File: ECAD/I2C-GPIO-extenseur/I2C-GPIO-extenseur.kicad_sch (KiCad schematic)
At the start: 61 parts, among them J1 Conn_01x03, J10 Conn_01x03, J11 Conn_01x03, J12 Conn_01x03, J13 Conn_01x03, J14 Conn_01x03, J15 Conn_01x03, J16 Conn_01x03, J17 Conn_01x03, J18 Conn_01x04, J19 Conn_01x04, J2 Conn_01x02, J3 Conn_01x03, J4 Conn_01x03, J5 Conn_01x03, J6 Conn_01x03, J7 Conn_01x03, J8 Conn_01x03, J9 Conn_01x03, U1 PCA9685PW

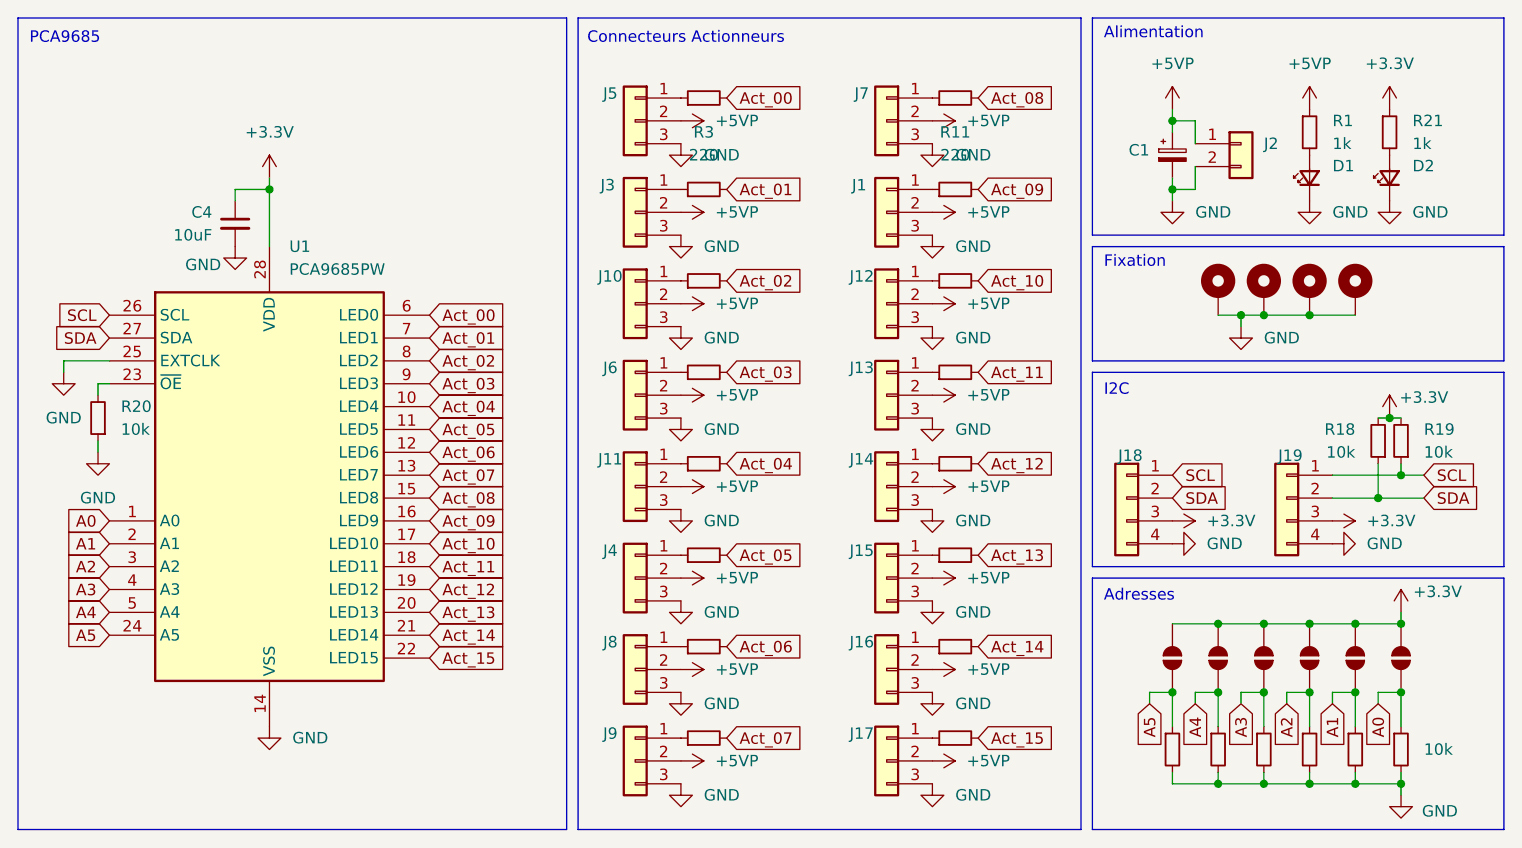
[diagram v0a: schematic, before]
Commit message: Attiny3216
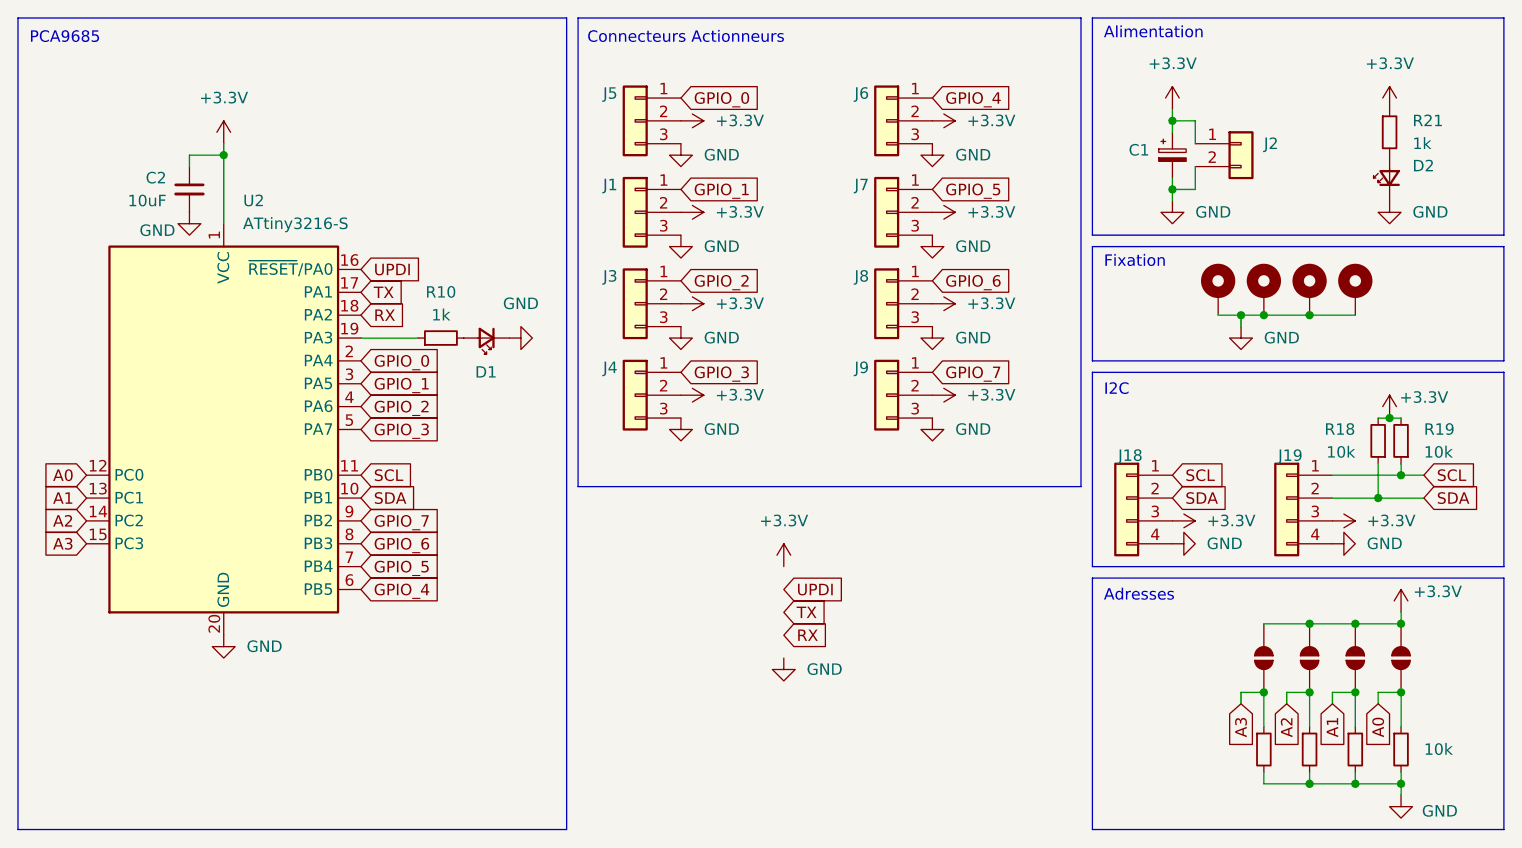
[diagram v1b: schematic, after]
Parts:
- removed C4: 10uF, Capacitor_SMD:C_1206_3216Metric_Pad1.33x1.80mm_HandSolder, symbol Device:C_Small
- removed J10, J11, J12, J13, J14, J15, J16, J17: Conn_01x03, Connector_PinHeader_2.54mm:PinHeader_1x03_P2.54mm_Vertical, symbol Connector_Generic:Conn_01x03
- removed JP5, JP6: SolderJumper_2_Open, Jumper:SolderJumper-2_P1.3mm_Open_RoundedPad1.0x1.5mm, symbol Jumper:SolderJumper_2_Open
- removed R11, R12, R13, R14, R15, R16, R17, R2, R3, R4, R5, R6, R7, R8, R9: 220, Resistor_SMD:R_1206_3216Metric_Pad1.30x1.75mm_HandSolder, symbol Device:R_Small
- removed R20, R25, R26, R27: 10k, Resistor_SMD:R_1206_3216Metric_Pad1.30x1.75mm_HandSolder, symbol Device:R_Small
- removed U1: PCA9685PW, Package_SO:TSSOP-28_4.4x9.7mm_P0.65mm, symbol Driver_LED:PCA9685PW
- added C2: 10uF, Capacitor_SMD:C_1206_3216Metric_Pad1.33x1.80mm_HandSolder, symbol Device:C_Small
- added U2: ATtiny3216-S, Package_SO:SOIC-20W_7.5x12.8mm_P1.27mm, symbol MCU_Microchip_ATtiny:ATtiny3216-S
- R1: value 1k -> 10k
- R10: value 220 -> 1k
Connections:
- net Act_08 is gone; now on an unnamed net: R10.2
- net +3.3V: now also C1.1, J1.2 (Pin_2), J2.1 (Pin_1), J3.2 (Pin_2), J4.2 (Pin_2), J5.2 (Pin_2), J6.2 (Pin_2), J7.2 (Pin_2), J8.2 (Pin_2), J9.2 (Pin_2), C2.1, U2.1 (VCC)
- net A0: now also U2.12 (PC0)
- net A1: now also U2.13 (PC1)
- net A2: now also U2.14 (PC2)
- net A3: now also R1.1, U2.15 (PC3)
- net GND: now also R1.2, C2.2, U2.20 (GND)
- net SCL: now also U2.11 (PB0)
- net SDA: now also U2.10 (PB1)
- net GPIO_0: now reaches J5.1 (Pin_1)
- net GPIO_0: now also U2.2 (PA4)
- net GPIO_3: now reaches J4.1 (Pin_1)
- net GPIO_3: now also U2.5 (PA7)
- net at D1.2 (A): no longer R1.2
- net GPIO_6: now reaches J8.1 (Pin_1)
- net GPIO_6: now also U2.8 (PB3)
- net GPIO_7: now reaches J9.1 (Pin_1)
- net GPIO_7: now also U2.9 (PB2)
- net at R10.1: now also U2.19 (PA3); no longer J7.1 (Pin_1)
- net GPIO_4: now reaches J6.1 (Pin_1)
- net GPIO_4: now also U2.6 (PB5)
- net GPIO_1: now reaches J1.1 (Pin_1)
- net GPIO_1: now also U2.3 (PA5)
- net GPIO_2: now reaches J3.1 (Pin_1)
- net GPIO_2: now also U2.4 (PA6)
- removed net +5VP: C1.1, J1.2 (Pin_2), J2.1 (Pin_1), J3.2 (Pin_2), J4.2 (Pin_2), J5.2 (Pin_2), J6.2 (Pin_2), J7.2 (Pin_2), J8.2 (Pin_2), J9.2 (Pin_2), R1.1
- new net GPIO_5: J7.1 (Pin_1), U2.7 (PB4)
- new net RX: U2.18 (PA2)
- new net TX: U2.17 (PA1)
- new net UPDI: U2.16 (~{RESET}/PA0)

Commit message: update size and position
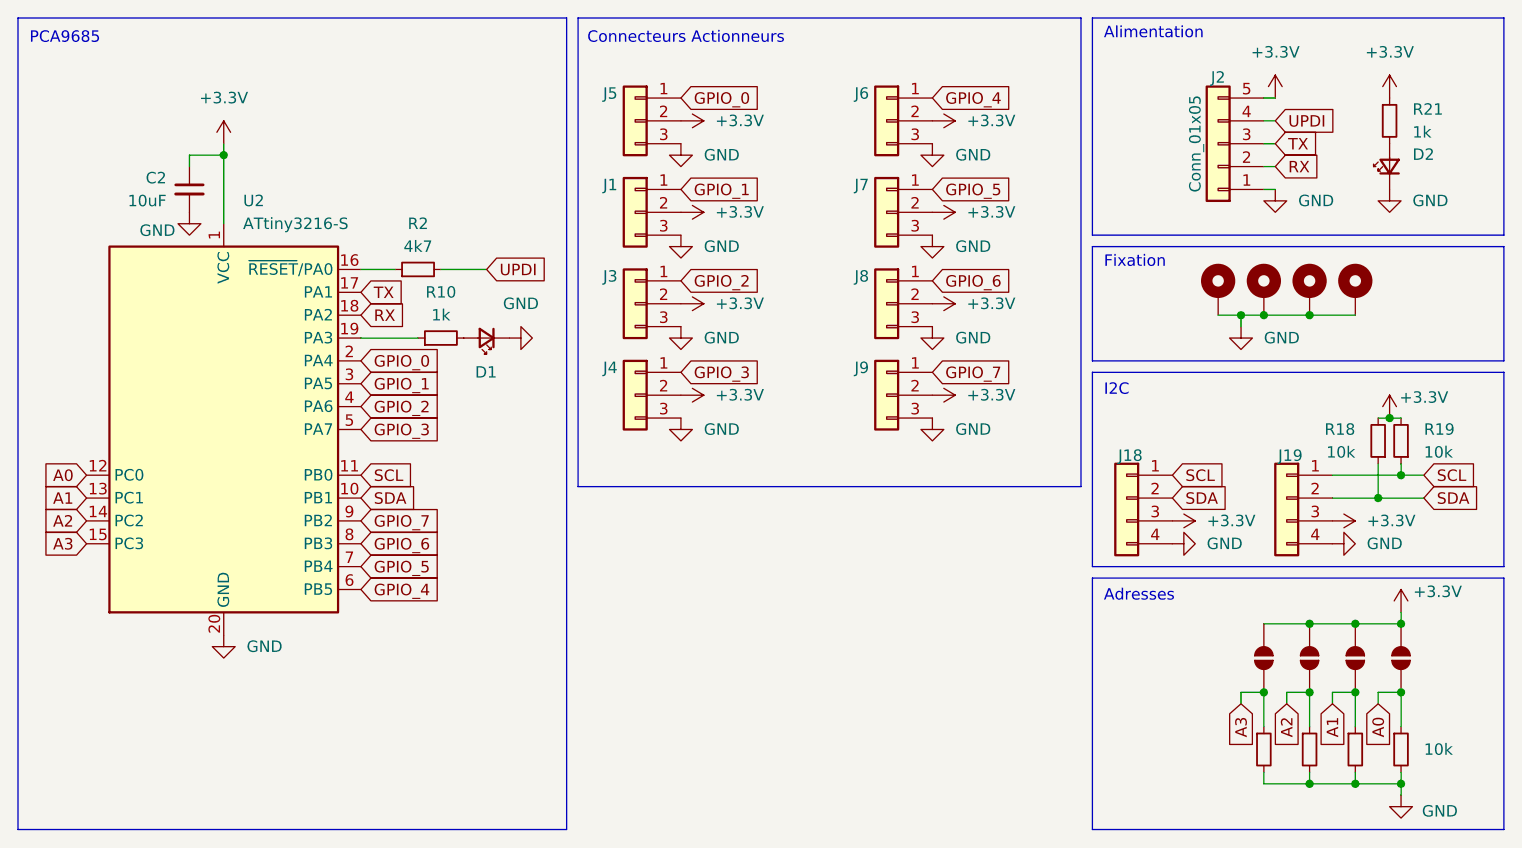
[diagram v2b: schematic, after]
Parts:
- removed C1: C_Polarized_Small, Capacitor_THT:CP_Radial_D10.0mm_P5.00mm, symbol Device:C_Polarized_Small
- removed J2: Conn_01x02, Connector_Molex:Molex_KK-396_A-41791-0002_1x02_P3.96mm_Vertical, symbol Connector_Generic:Conn_01x02
- added J2: Conn_01x05, Connector_PinHeader_2.54mm:PinHeader_1x05_P2.54mm_Vertical, symbol Connector_Generic:Conn_01x05
- added R2: 4k7, Resistor_SMD:R_1206_3216Metric_Pad1.30x1.75mm_HandSolder, symbol Device:R_Small
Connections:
- net +3.3V: now also J2.5 (Pin_5)
- net GND: now also J2.1 (Pin_1)
- net RX: now also J2.2 (Pin_2)
- net TX: now also J2.3 (Pin_3)
- net UPDI: now also J2.4 (Pin_4), R2.2; no longer U2.16 (~{RESET}/PA0)
- new net: R2.1, U2.16 (~{RESET}/PA0)
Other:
- moved on the sheet: D2, R21
